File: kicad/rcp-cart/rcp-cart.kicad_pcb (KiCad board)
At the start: 2 copper layers, 106.3 x 22.9 mm, 4 parts, among them P5 CART-EDGE

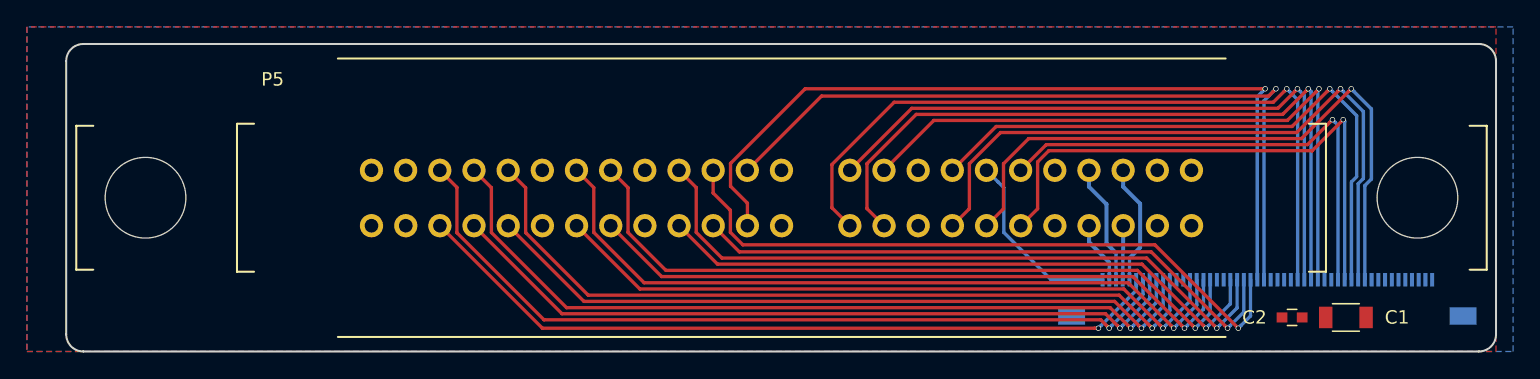
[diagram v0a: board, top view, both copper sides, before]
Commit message: Almost done
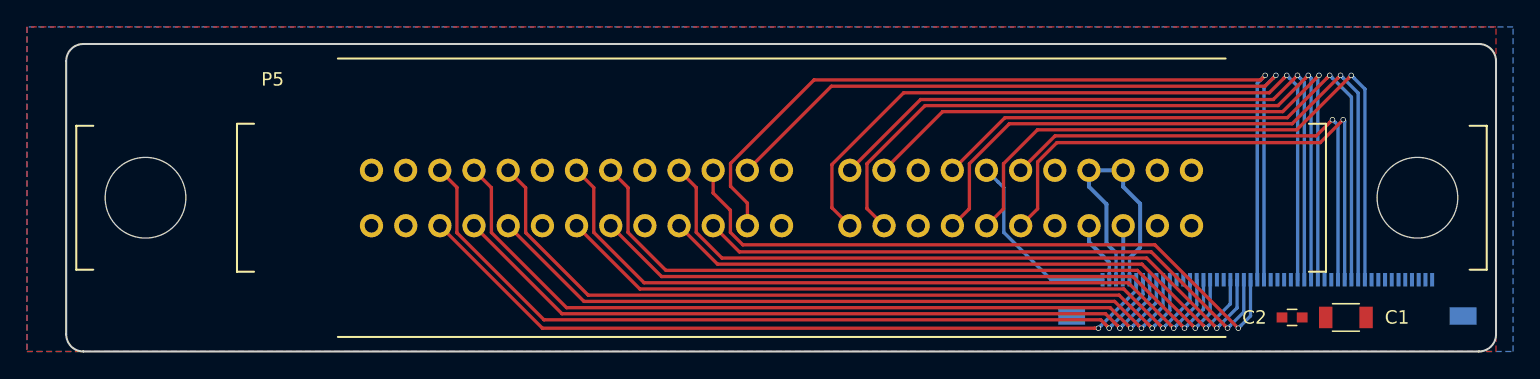
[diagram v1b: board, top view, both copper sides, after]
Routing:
- net GND: track 27.2 -> 29.8 mm
- net /CART_ADDR10: track 61.6 -> 63.1 mm
- net /CART_ADDR08: track 54.5 -> 56.0 mm
- net /CART_ADDR07: track 49.1 -> 50.5 mm
- net /CART_ADDR09: track 55.8 -> 57.2 mm
- net /CART_ADDR06: track 50.2 -> 51.6 mm
- net /CART_ADDR05: track 56.4 -> 57.8 mm
- net /PIF_CIC_DAT_OUT: track 50.1 -> 51.2 mm
- net /PIF_CIC_DAT_IN: track 45.8 -> 46.8 mm
- net /CIC_CLK: track 48.3 -> 49.3 mm
